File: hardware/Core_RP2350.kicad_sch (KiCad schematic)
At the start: 73 parts, among them J1 5-146281-3, J2 5-146281-3, J3 AudioJack3, J4 USB_C_Receptacle_USB2.0, J5 Micro_SD_Card_Det_Hirose_DM3AT, SW1 SPST-NO, SW2 SPST-NO, SW3 SPST-NO, U2 W25Q16JVUXIQ, U3 ADUM4160, U32 RP2350_80QFN

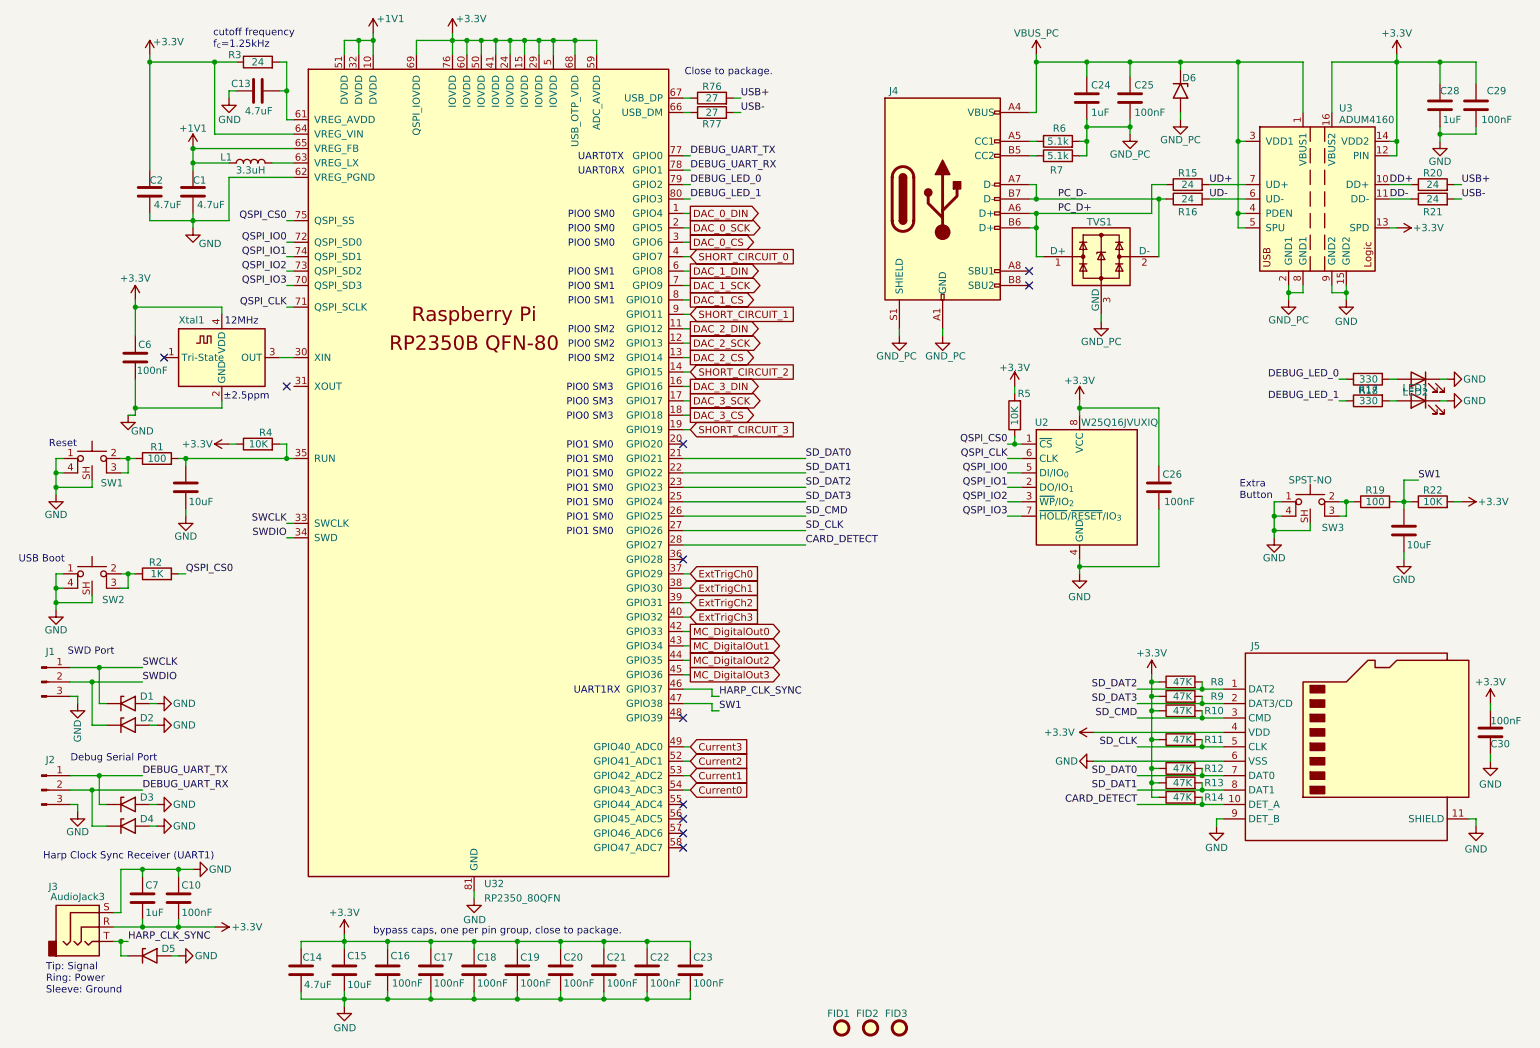
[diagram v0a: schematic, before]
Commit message: update pcb draft
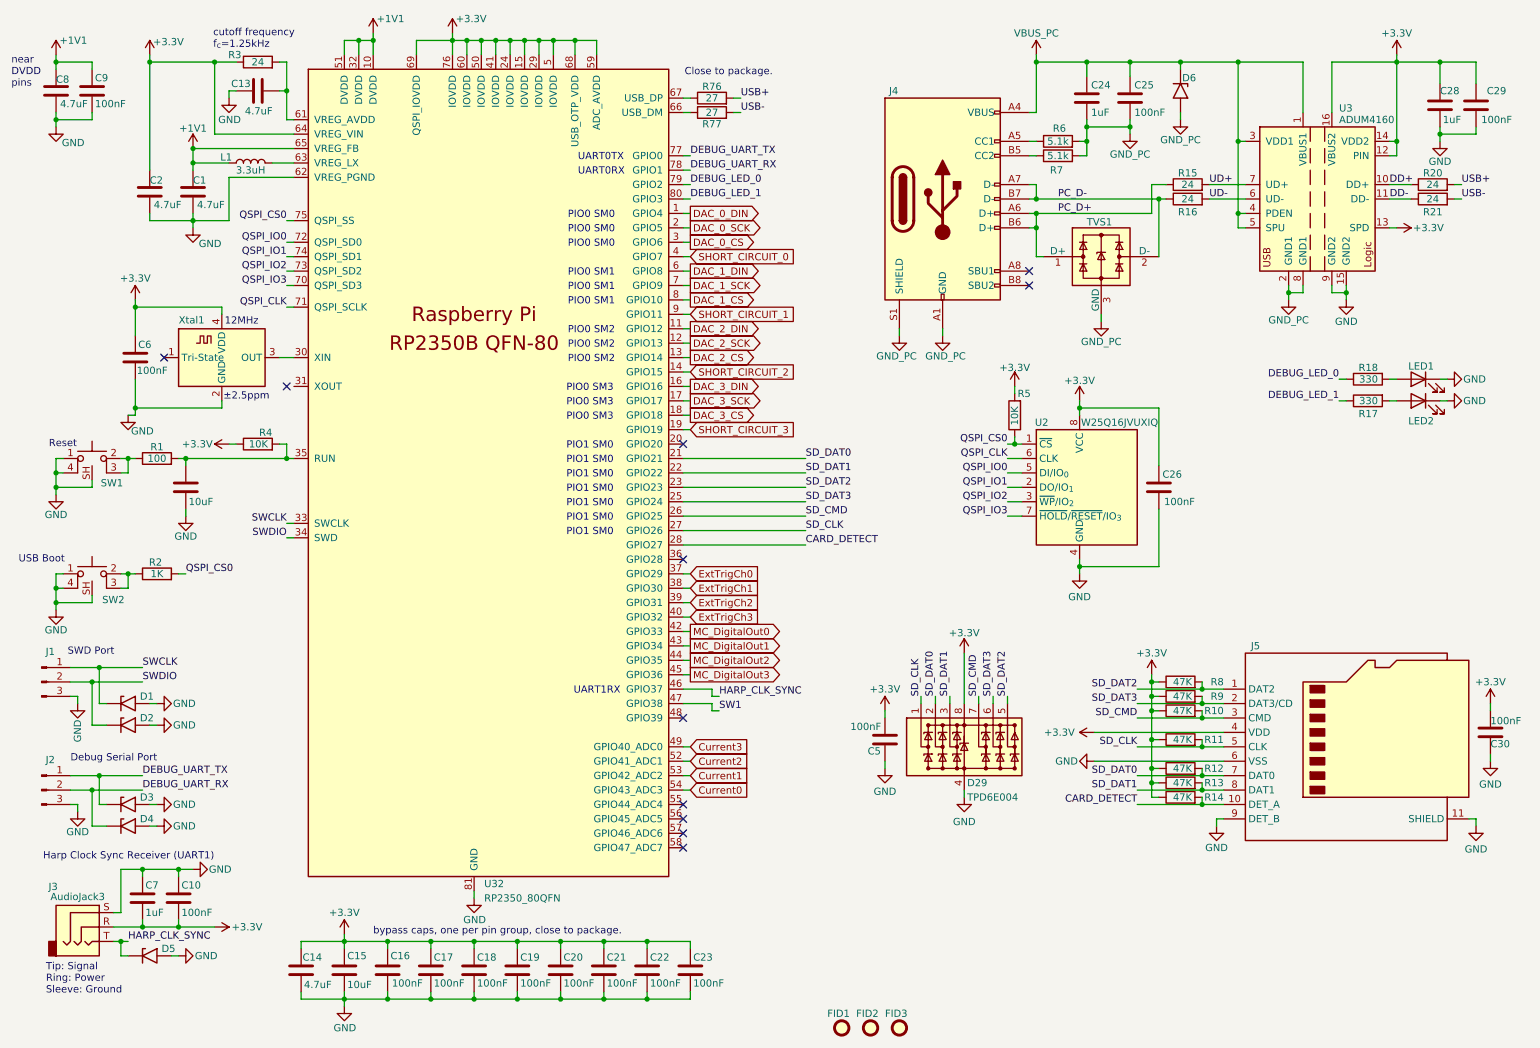
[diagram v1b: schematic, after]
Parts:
- removed C4: 10uF, Capacitor_SMD:C_0603_1608Metric, symbol harp.device.quad.dac:C_0603
- removed R19: 100, Resistor_SMD:R_0603_1608Metric, symbol harp.device.quad.dac:R_0603
- removed R22: 10K, Resistor_SMD:R_0402_1005Metric, symbol harp.device.quad.dac:R_0603
- removed SW3: SPST-NO, kicad-lib:SW_Push_1P1T-SH_NO_Vertical_Wuerth_WS-TASV, symbol harp.device.quad.dac:SW_Push_with_gnd
- added C5, C9: 100nF, Capacitor_SMD:C_0402_1005Metric, symbol harp.device.quad.dac:C_0603
- added C8: 4.7uF, Capacitor_SMD:C_0603_1608Metric, symbol harp.device.quad.dac:C_0603
- added D29: TPD6E004, kicad-lib:IC_TPD6E004RSER, symbol kicad-lib:TPD6E004
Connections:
- net +1V1: now also C8.1, C9.2
- net +3.3V: now also C5.1, D29.8 (Vcc)
- net GND: now also C5.2, C8.2, C9.1, D29.4 (GND)
- net SD_CLK: now also D29.1 (K1)
- net SD_CMD: now also D29.7 (K6)
- net SD_DAT0: now also D29.2 (K2)
- net SD_DAT1: now also D29.3 (K3)
- net SD_DAT2: now also D29.5 (K4)
- net SD_DAT3: now also D29.6 (K5)
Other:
- note added: "near DVDD pins"
- note removed: "Extra Button"

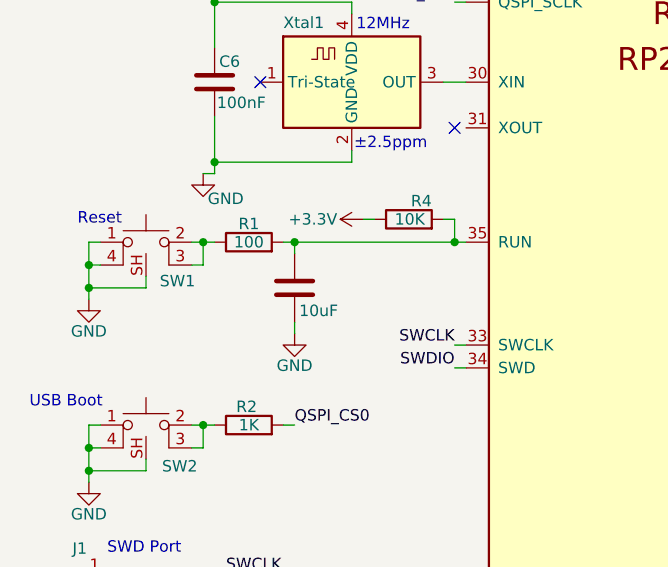
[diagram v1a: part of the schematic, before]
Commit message: update pcb
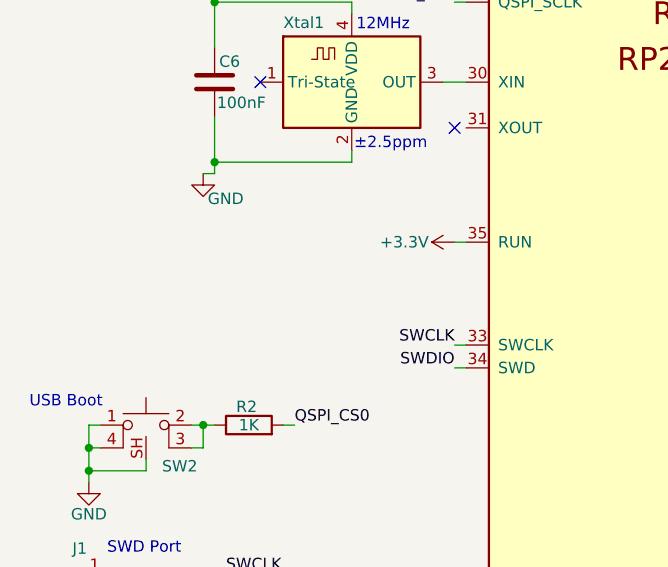
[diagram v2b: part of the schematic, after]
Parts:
- removed C3: 10uF, Capacitor_SMD:C_0603_1608Metric, symbol harp.device.quad.dac:C_0603
- removed R1: 100, Resistor_SMD:R_0603_1608Metric, symbol harp.device.quad.dac:R_0603
- removed R4: 10K, Resistor_SMD:R_0402_1005Metric, symbol harp.device.quad.dac:R_0603
- removed SW1: SPST-NO, kicad-lib:SW_Push_1P1T-SH_NO_Vertical_Wuerth_WS-TASV, symbol harp.device.quad.dac:SW_Push_with_gnd
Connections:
- net +3.3V: now also U32.35 (RUN)
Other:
- note removed: "Reset"
